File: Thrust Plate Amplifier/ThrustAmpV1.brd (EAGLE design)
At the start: 97.1 x 77.5 mm, 61 parts, among them U1 INA126PA, U2 INA126PA, U3 INA126PA, U4 INA126PA, U5 LP2985AIM5-3.3, U6 LP2985AIM5-5.0/NOPB

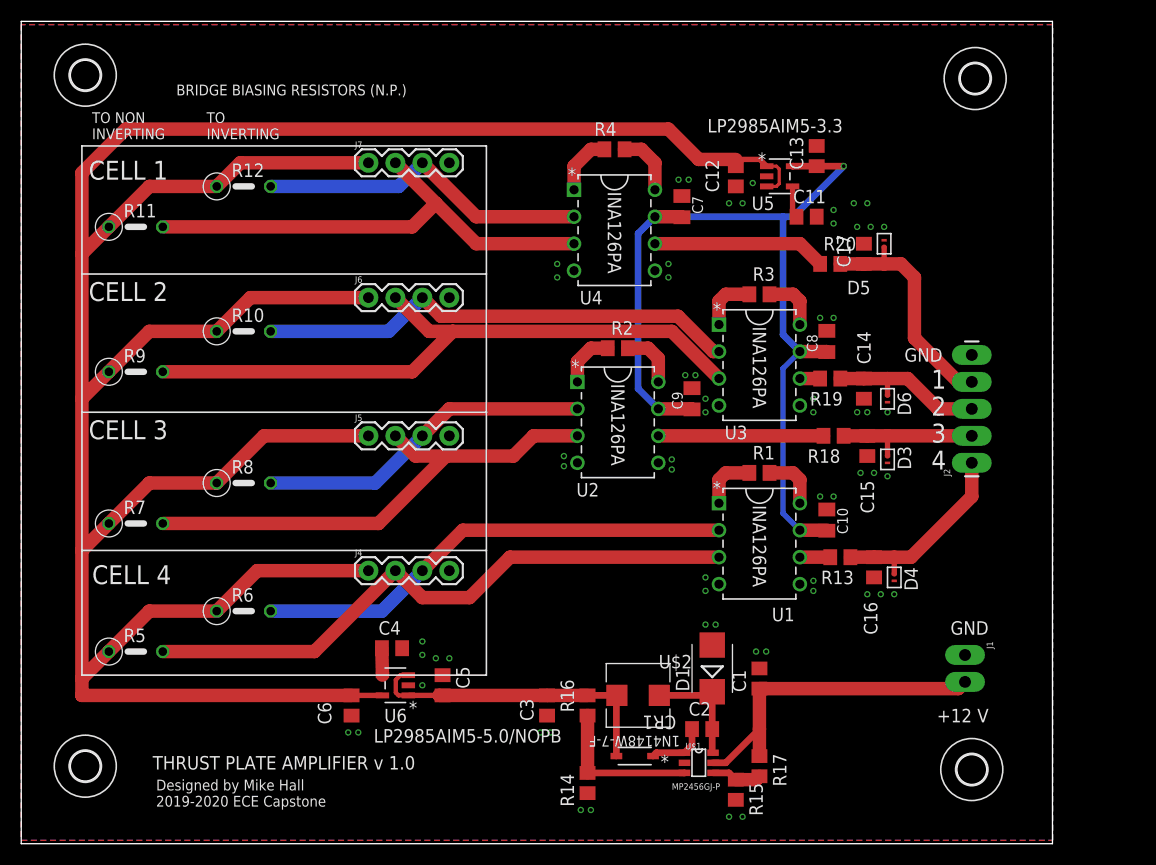
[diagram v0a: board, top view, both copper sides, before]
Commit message: THE PENULTIMATE AMPLIFIER
ALMOST ready for OSHpark. Just a few minor chores left.
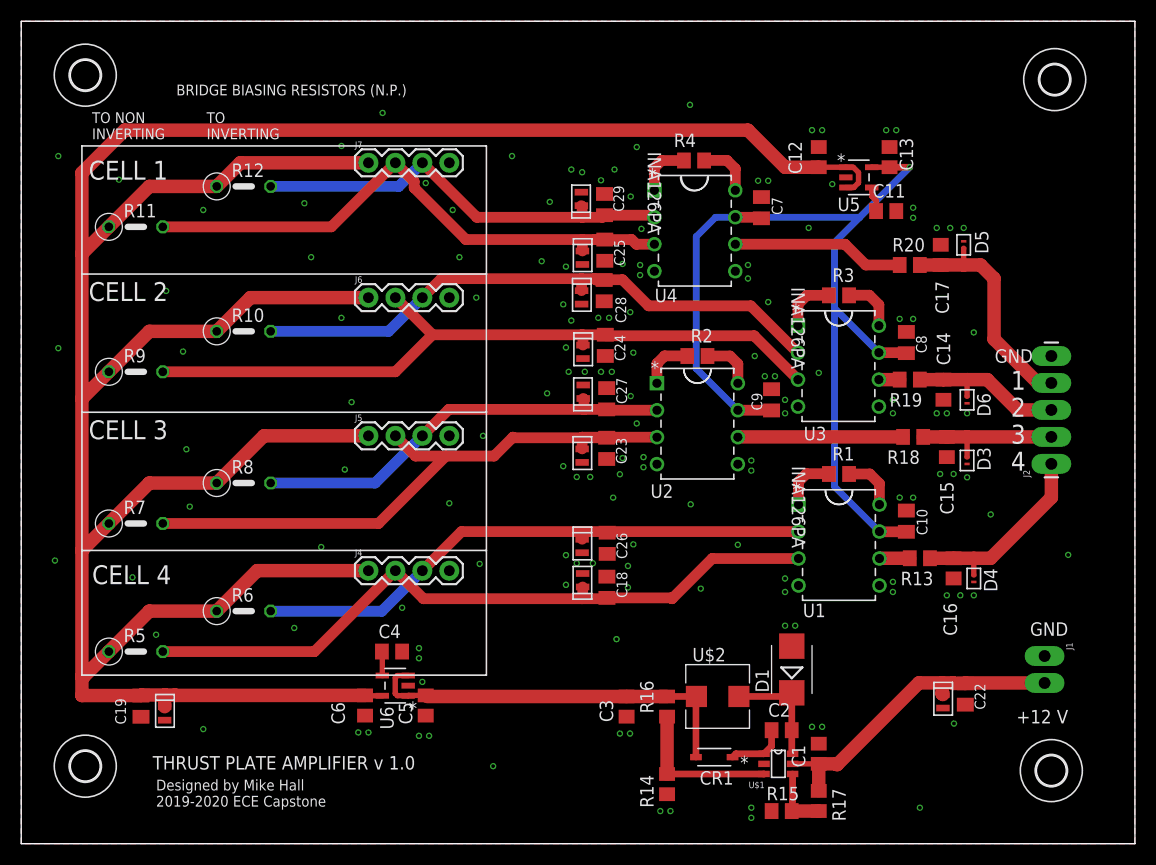
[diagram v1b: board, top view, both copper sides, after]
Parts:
- added C18, C23, C24, C25, C26, C27, C28, C29: 100 pF, rcl:C0805K
- added C19, C22: 100 nF, rcl:C0805K
- added D10, D11, D12, D13, D14, D15, D2, D7, D8, D9: (no value), D5V0H1U2LP1610-7:0603DIODE
- D1: value (none) -> 10BQ060TR
- moved C1 9.02 mm to (75.1, 8.47)
- moved C12 8.02 mm to (75.1, 64.7), turned to 90 degrees
- moved R4 7.57 mm to (63.4, 64.4)
- moved R2 7.53 mm to (63.7, 45.9)
- moved C11 7.51 mm to (81.5, 59.6)
- moved C10 7.49 mm to (83.4, 30.4)
- moved C15 7.49 mm to (87.2, 37.4)
- moved C8 7.49 mm to (83.4, 47.2)
- moved CR1 7.49 mm to (65.3, 8.15)
- moved D3 7.49 mm to (89.1, 36.1)
- moved D6 7.49 mm to (89.1, 41.8)
- moved H1 7.49 mm to (97.0, 6.88)
- moved J2 7.49 mm to (97.0, 35.8)
- moved C3 7.49 mm to (57.0, 12.9)
- moved C7 7.49 mm to (69.7, 59.9)
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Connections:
- net 12V: now also C22.1, D9.P$2
- net 5V: now also C19.1, D15.P$2
- net GND: now also C18.2, C19.2, C22.2, C23.2, C24.2, C25.2, C26.2, C27.2, C28.2, C29.2, D10.P$1, D11.P$1, D12.P$1, D13.P$1, D14.P$1, D15.P$1, D2.P$1, D7.P$1, D8.P$1, D9.P$1
- net N$100: now also C29.1, D2.P$2
- net N$93: now also C18.1, D11.P$2
- net N$94: now also C26.1, D10.P$2
- net N$95: now also C23.1, D12.P$2
- net N$96: now also C27.1, D8.P$2
- net N$97: now also C24.1, D13.P$2
- net N$98: now also C28.1, D7.P$2
- net N$99: now also C25.1, D14.P$2
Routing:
- net N$95: track 48.0 -> 59.0 mm
- net N$98: track 45.6 -> 55.8 mm
- net N$93: track 58.2 -> 67.0 mm
- net N$100: track 31.6 -> 40.5 mm
- net N$96: track 31.8 -> 40.3 mm
- net N$94: track 45.4 -> 53.7 mm
- net 5V: track 273.9 -> 281.5 mm
- net 6V: track 29.5 -> 37.1 mm
- net N$99: track 46.6 -> 53.4 mm
- net 3.3V: track 87.0 -> 93.5 mm
- net N$97: track 62.5 -> 69.0 mm
- net N$28: track 4.77 -> 6.04 mm
- net 12V: track 31.7 -> 30.7 mm
- net N$7: track 5.93 -> 5.30 mm
- net N$25: track 3.01 -> 2.39 mm
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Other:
- board size 97.1 x 77.5 mm -> 104.9 x 77.5 mm
